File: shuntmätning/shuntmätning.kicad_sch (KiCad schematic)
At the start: 10 parts, among them U1 MCP6002-xP, U2 MCP6002-xP

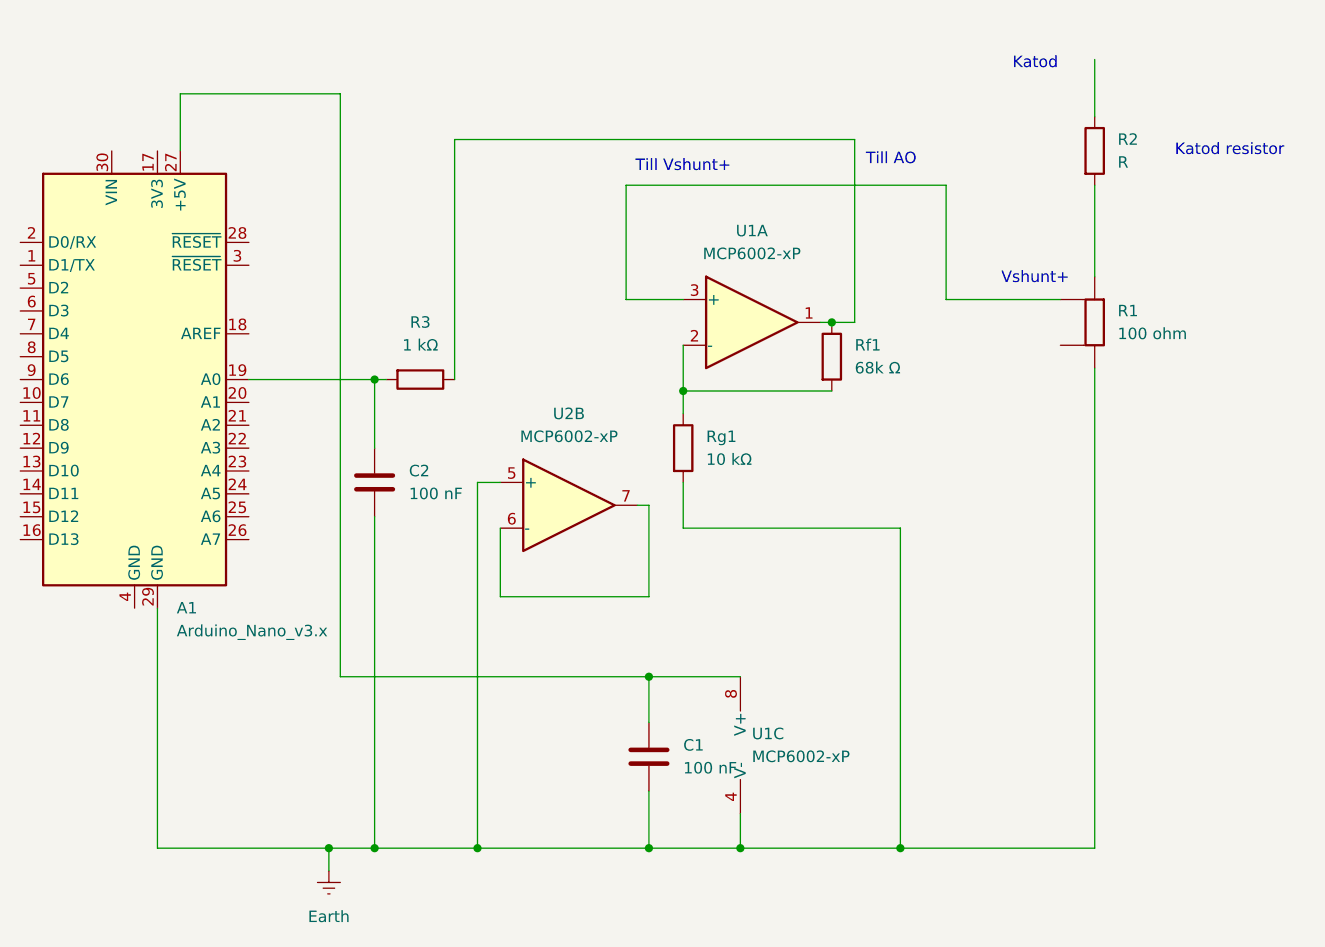
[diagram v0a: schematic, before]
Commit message: Lägg till hela my_kicad_work
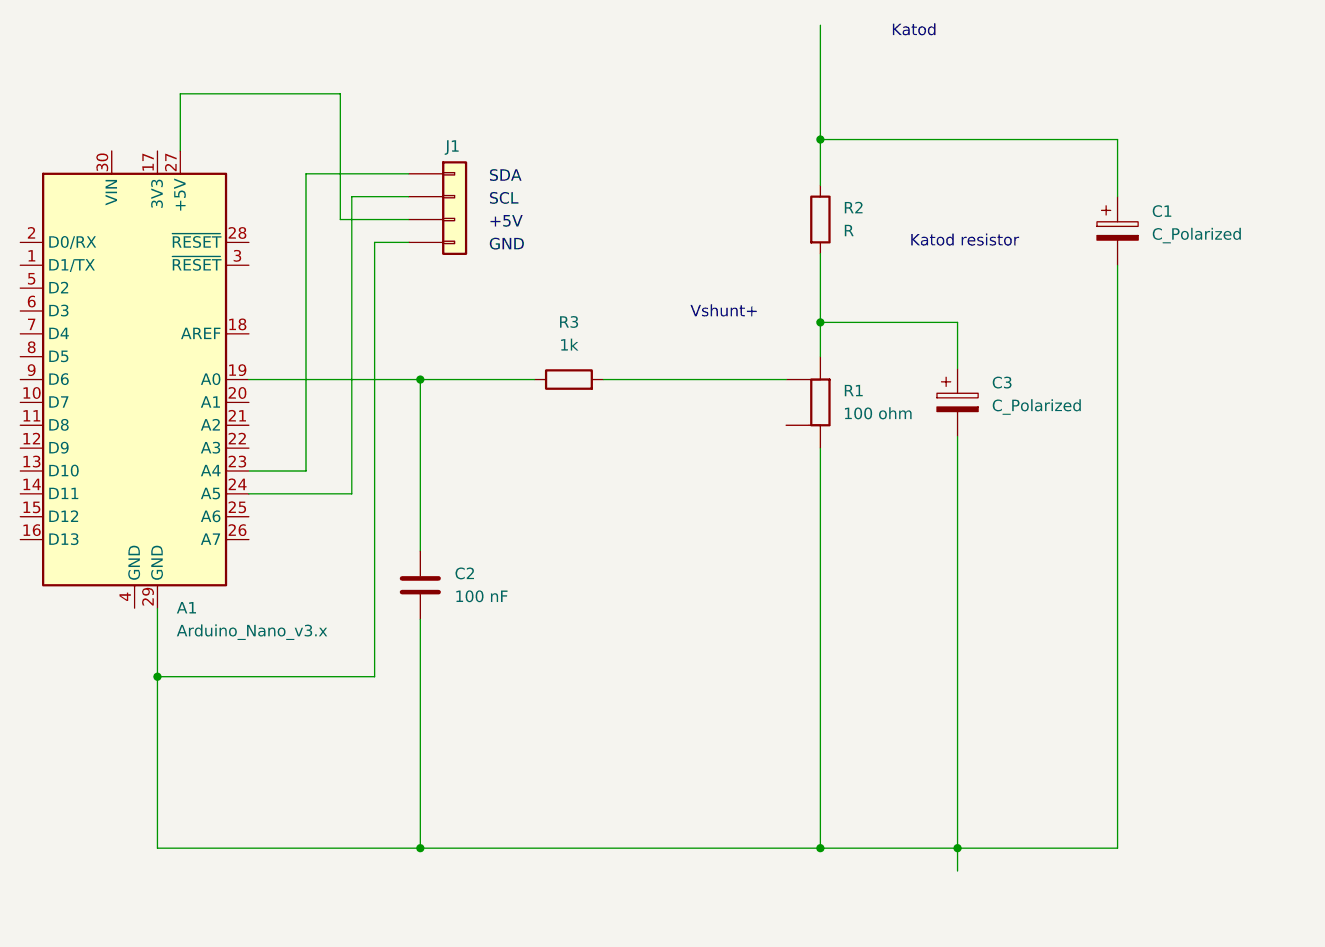
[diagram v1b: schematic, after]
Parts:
- removed C1: 100 nF, Capacitor_THT:CP_Axial_L37.0mm_D16.0mm_P43.00mm_Horizontal, symbol Device:C
- removed Rf1: 68k Ω, Resistor_THT:R_Axial_DIN0204_L3.6mm_D1.6mm_P7.62mm_Horizontal, symbol Device:R
- removed Rg1: 10 kΩ, Resistor_THT:R_Axial_DIN0204_L3.6mm_D1.6mm_P7.62mm_Horizontal, symbol Device:R
- removed U1, U2: MCP6002-xP, Button_Switch_SMD:SW_DIP_SPSTx04_Slide_6.7x11.72mm_W6.73mm_P2.54mm_LowProfile_JPin, symbol Amplifier_Operational:MCP6002-xP
- added C1, C3: C_Polarized, symbol Device:C_Polarized
- added J1: ~, symbol Connector_Generic:Conn_01x04
- C2: footprint Capacitor_THT:CP_Axial_L37.0mm_D16.0mm_P43.00mm_Horizontal -> (none)
- R3: value 1 kΩ -> 1k
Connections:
- net at R3.1: now also A1.19 (A0), C2.1
- net at A1.23 (A4): now also J1.1 (Pin_1)
- net at A1.24 (A5): now also J1.2 (Pin_2)
- net at A1.27 (+5V): now also J1.3 (Pin_3)
- net at R1.3: now also R3.2
- net at R2.1: now also C1.1
- net at R1.4, R2.2: now also C3.1
- net Earth: no longer names the net of A1.29 (GND), C2.2, R1.1
- net Earth: now also C1.2, C3.2, J1.4 (Pin_4)
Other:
- note removed: "Till AO"
- note removed: "Till Vshunt+"
- moved on the sheet: R1, R2
